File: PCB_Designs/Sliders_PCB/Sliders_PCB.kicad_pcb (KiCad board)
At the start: 2 copper layers, 67.1 x 83.6 mm, 10 parts, among them P1 CONN_02X05, P2 CONN_01X01, P3 CONN_01X01, P4 CONN_01X01, P5 CONN_01X01

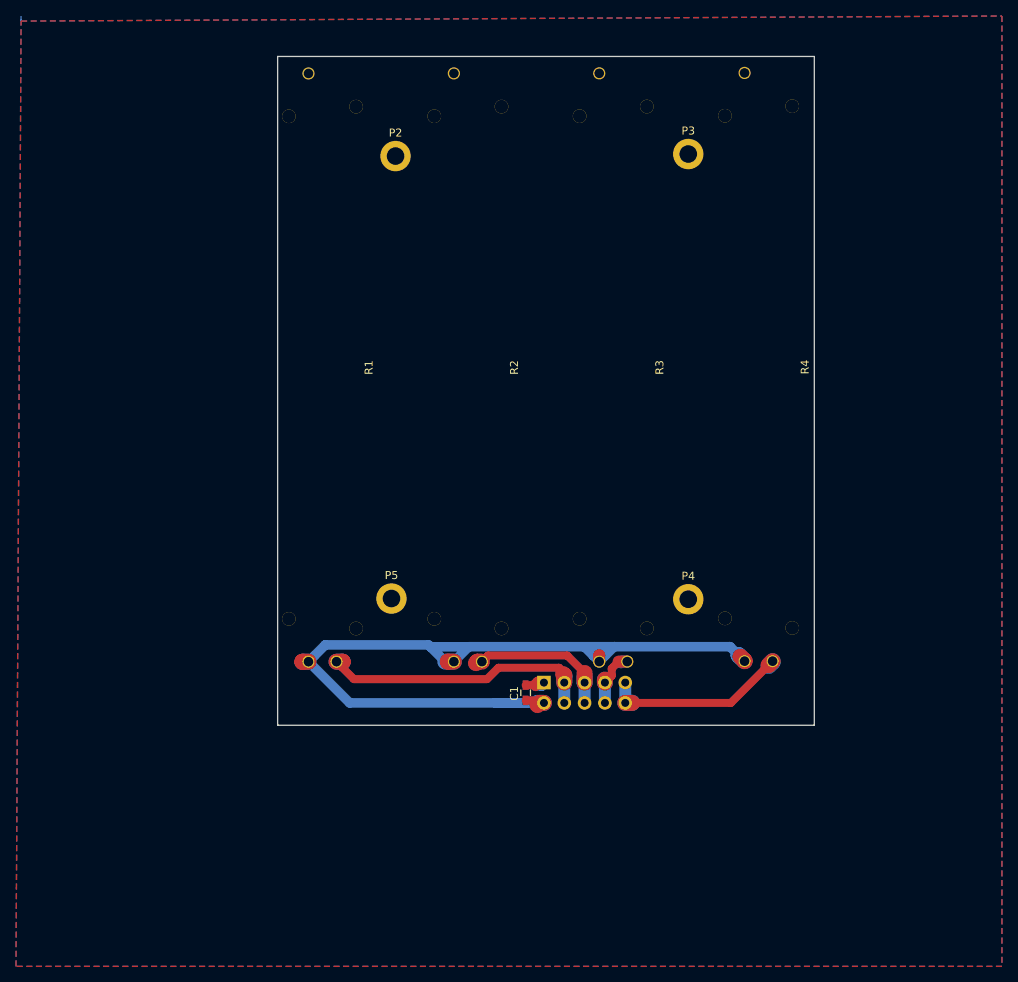
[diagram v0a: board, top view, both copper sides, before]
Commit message: Manufacture files added
* Gerbers created
* Drillfiles created
* G-CODE generated (milling information)
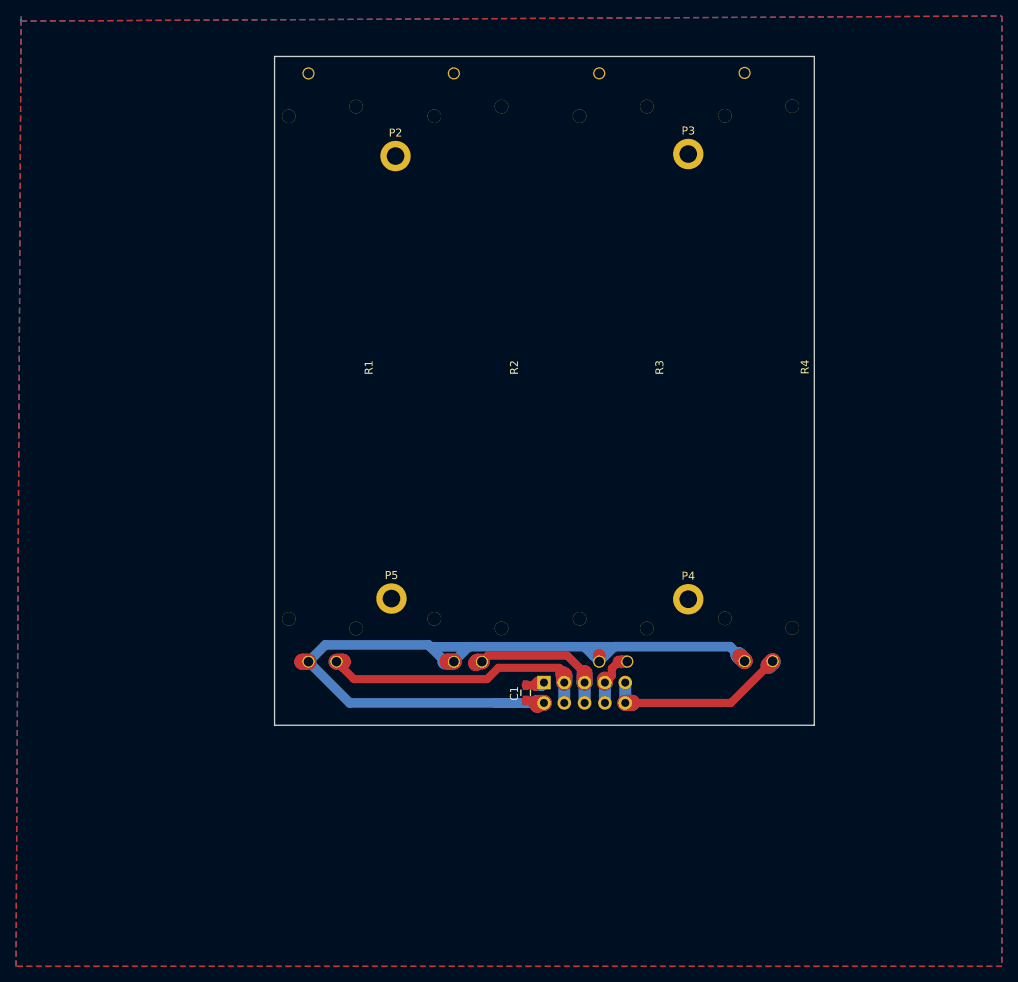
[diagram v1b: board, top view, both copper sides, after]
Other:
- board size 67.1 x 83.6 mm -> 67.4 x 83.6 mm
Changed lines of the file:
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@@
     (area 66.675 18.806699 189.865001 139.700001)
     (thickness 1.6)
-    (drawings 10)
+    (drawings 7)
     (tracks 89)
     (zones 0)
@@
   )
   (setup
-    (last_trace_width 1.5)
+    (last_trace_width 0.7)
     (user_trace_width 0.7)
     (user_trace_width 0.8)
@@
     (pad_drill 0.762)
     (pad_to_mask_clearance 0.2)
-    (aux_axis_origin 0 0)
-    (grid_origin 106.7308 101.9556)
+    (aux_axis_origin 98.9908 109.5756)
+    (grid_origin 98.9908 109.5756)
     (visible_elements 7FFFFFFF)
     (pcbplotparams
-      (layerselection 0x00000_00000001)
+      (layerselection 0x01000_80000001)
       (usegerberextensions false)
       (excludeedgelayer true)
@@
       (viasonmask false)
       (mode 1)
-      (useauxorigin false)
+      (useauxorigin true)
       (hpglpennumber 1)
       (hpglpenspeed 20)
@@
       (psnegative false)
       (psa4output false)
-      (plotreference true)
-      (plotvalue true)
+      (plotreference false)
+      (plotvalue false)
       (plotinvisibletext false)
       (padsonsilk false)
@@
       (drillshape 0)
       (scaleselection 1)
-      (outputdirectory ""))
+      (outputdirectory ../GERBERS/Sliders_PCB/))
   )
   (net 0 "")
@@
       (net 10 "Net-(P5-Pad1)"))
   )
-  (target plus (at 76.095017 25.913497) (size 5) (width 0.15) (layer Edge.Cuts))
-  (target plus (at 183.028766 26.0356) (size 5) (width 0.15) (layer Edge.Cuts))
-  (target plus (at 181.457411 109.60964) (size 5) (width 0.15) (layer Edge.Cuts))
   (dimension 83.435672 (width 0.3) (layer F.SilkS)
     (gr_text "83,436 mm" (at 171.834915 67.778236 90) (layer F.SilkS)
@@
     (arrow2b (pts (xy 109.382079 21.608134) (xy 110.502035 21.009302)))
   )
-  (gr_line (start 166.4208 26.0096) (end 99.3648 26.0096) (layer Edge.Cuts) (width 0.15))
+  (gr_line (start 166.4208 26.0096) (end 98.980796 26.0096) (layer Edge.Cuts) (width 0.15))
   (gr_line (start 166.4208 109.5756) (end 166.4208 26.0096) (layer Edge.Cuts) (width 0.15))
-  (gr_line (start 99.3648 109.5756) (end 166.4208 109.5756) (layer Edge.Cuts) (width 0.15))
-  (gr_line (start 99.3648 26.0096) (end 99.3648 109.5756) (layer Edge.Cuts) (width 0.15))
+  (gr_line (start 98.980794 109.5756) (end 166.4208 109.5756) (layer Edge.Cuts) (width 0.15))
+  (gr_line (start 98.9808 26.0056) (end 98.9808 109.575701) (layer Edge.Cuts) (width 0.15))
   (dimension 67.31 (width 0.3) (layer F.SilkS)
     (gr_text 67,310mm (at 132.715 24.685) (layer F.SilkS)
